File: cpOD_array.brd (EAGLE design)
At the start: 128.3 x 106.7 mm, 189 parts, among them IC1X11 LM358D, IC1X12 LM358D, IC1X13 LM358D, IC1X21 LM358D, IC1X22 LM358D, IC1X23 LM358D, Q1X11 2N7002, Q1X12 2N7002, Q1X13 2N7002, Q1X21 2N7002, Q1X22 2N7002, Q1X23 2N7002

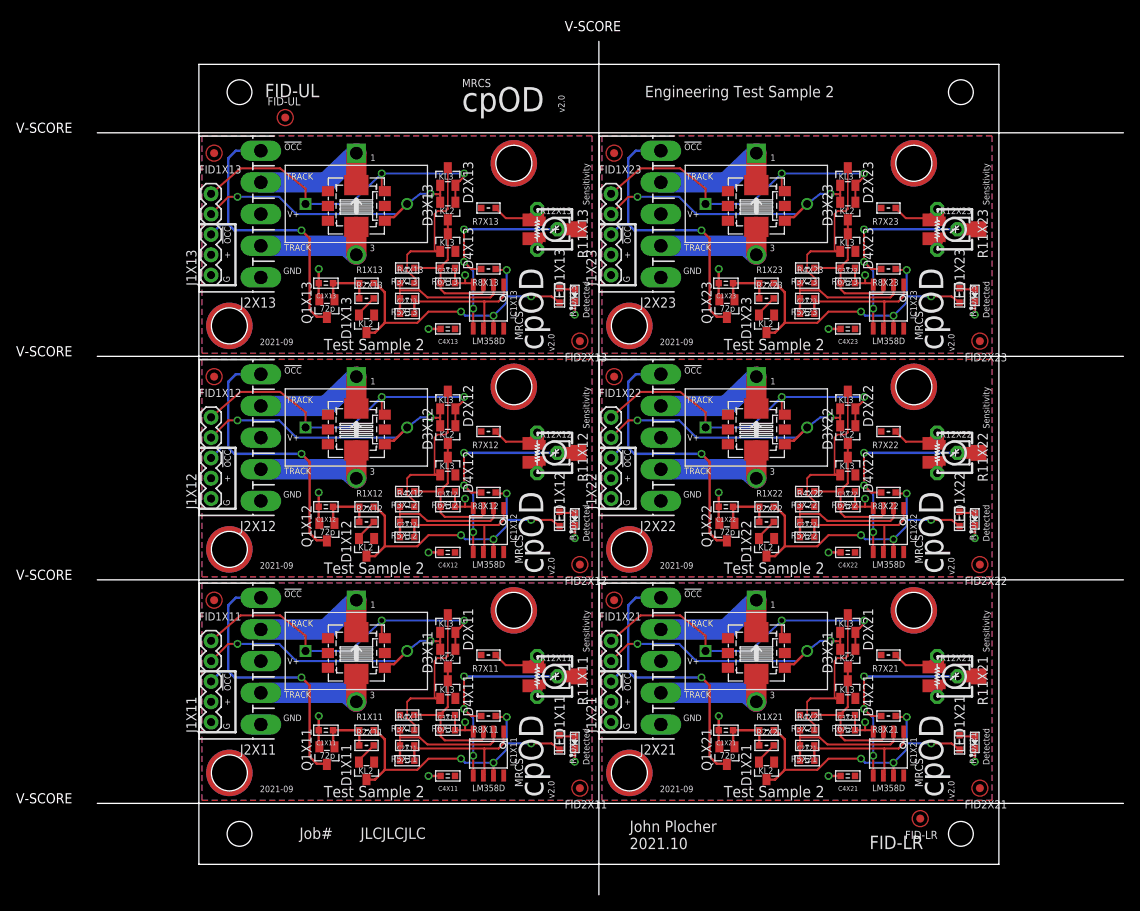
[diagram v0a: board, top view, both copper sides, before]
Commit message: panelized
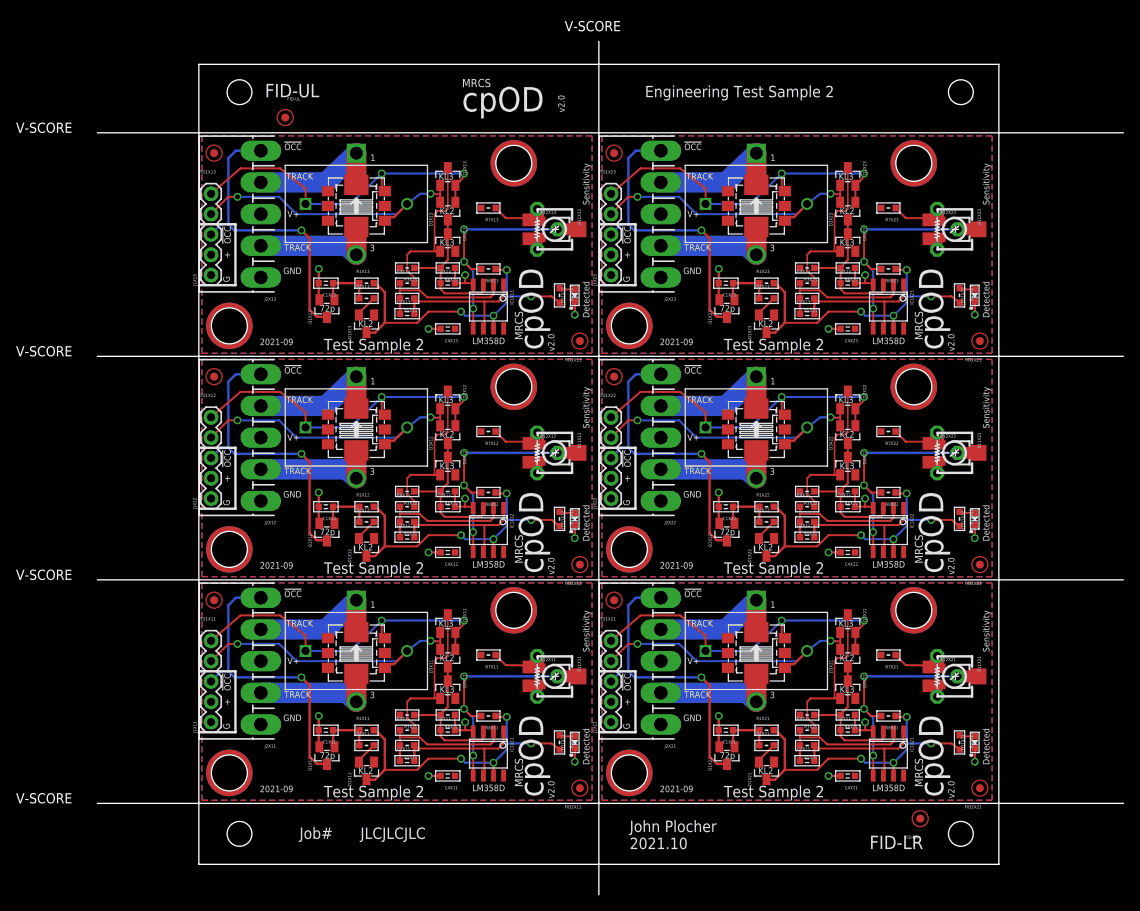
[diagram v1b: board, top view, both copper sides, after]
